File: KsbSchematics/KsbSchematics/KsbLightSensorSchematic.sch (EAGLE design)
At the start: 32 parts, among them IC1 7805L, IC2 LM311N, U1 ATTINY84

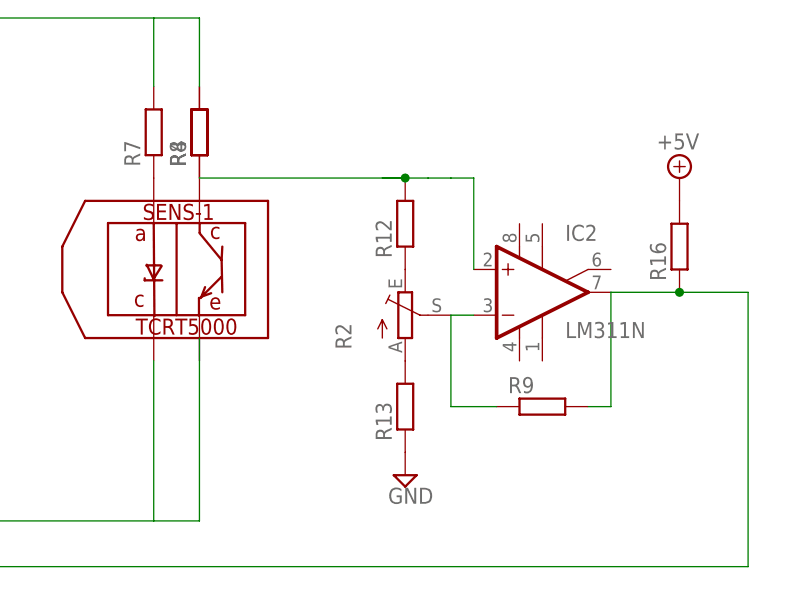
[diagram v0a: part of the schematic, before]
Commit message: minor changes
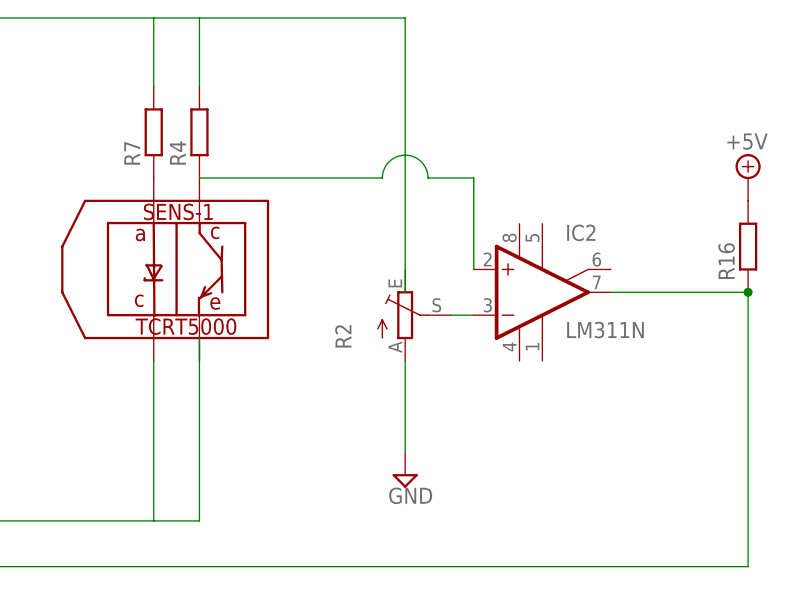
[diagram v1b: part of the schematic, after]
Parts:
- removed R12, R13, R8, R9: (no value), resistor:R-EU_0613/5V
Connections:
- removed net N$14: R4.1, R8.1
- removed net N$17: R12.1, R2.E
- removed net N$18: R13.2, R2.A
- removed net N$7: IC2.-IN, R2.S, R9.1
- new net N$21: IC2.+IN, SENS-1.P$1
- net +12V: no longer R8.2
- net GND: now also R2.A; no longer R13.1
- net N$13: now also IC2.-IN, R2.S; no longer IC2.+IN, R12.2, R8.1, SENS-1.P$1
- net N$4: no longer R9.2
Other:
- moved on the sheet: R16
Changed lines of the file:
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@@
 <part name="R4" library="resistor" deviceset="R-EU_" device="0613/5V"/>
 <part name="R7" library="resistor" deviceset="R-EU_" device="0613/5V"/>
-<part name="R8" library="resistor" deviceset="R-EU_" device="0613/5V"/>
-<part name="R9" library="resistor" deviceset="R-EU_" device="0613/5V"/>
 <part name="R10" library="resistor" deviceset="R-EU_" device="0613/5V" value="2k"/>
 <part name="R11" library="resistor" deviceset="R-EU_" device="0613/5V" value="2k"/>
@@
 <part name="SUPPLY8" library="supply2" deviceset="GND" device=""/>
 <part name="SUPPLY11" library="supply2" deviceset="GND" device=""/>
-<part name="R12" library="resistor" deviceset="R-EU_" device="0613/5V"/>
-<part name="R13" library="resistor" deviceset="R-EU_" device="0613/5V"/>
 <part name="SUPPLY6" library="supply2" deviceset="GND" device=""/>
 <part name="SG1" library="buzzer" deviceset="EFB?" device="AA40D101"/>
@@
 <instance part="R4" gate="G$1" x="93.98" y="152.4" rot="R90"/>
 <instance part="R7" gate="G$1" x="88.9" y="152.4" rot="R90"/>
-<instance part="R8" gate="G$1" x="93.98" y="152.4" rot="R90"/>
-<instance part="R9" gate="G$1" x="132.08" y="121.92"/>
 <instance part="R10" gate="G$1" x="-15.24" y="86.36"/>
 <instance part="R11" gate="G$1" x="-15.24" y="48.26"/>
@@
 <instance part="SUPPLY8" gate="GND" x="-63.5" y="81.28"/>
 <instance part="SUPPLY11" gate="GND" x="-66.04" y="43.18"/>
-<instance part="R12" gate="G$1" x="116.84" y="142.24" rot="R90"/>
-<instance part="R13" gate="G$1" x="116.84" y="121.92" rot="R90"/>
 <instance part="SUPPLY6" gate="GND" x="116.84" y="114.3"/>
 <instance part="SG1" gate="G$1" x="106.68" y="86.36"/>
@@
 <instance part="SUPPLY21" gate="GND" x="10.16" y="0"/>
 <instance part="R15" gate="G$1" x="-12.7" y="7.62"/>
-<instance part="R16" gate="G$1" x="147.32" y="139.7" rot="R90"/>
-<instance part="SUPPLY22" gate="+12V" x="147.32" y="147.32"/>
+<instance part="R16" gate="G$1" x="154.94" y="139.7" rot="R90"/>
+<instance part="SUPPLY22" gate="+12V" x="154.94" y="147.32"/>
 </instances>
 <busses>
@@
 <wire x1="35.56" y1="124.46" x2="35.56" y2="165.1" width="0.1524" layer="91"/>
 <pinref part="R4" gate="G$1" pin="2"/>
-<pinref part="R8" gate="G$1" pin="2"/>
 <wire x1="93.98" y1="165.1" x2="93.98" y2="157.48" width="0.1524" layer="91"/>
 <wire x1="35.56" y1="165.1" x2="88.9" y2="165.1" width="0.1524" layer="91"/>
@@
 <pinref part="R7" gate="G$1" pin="2"/>
 <wire x1="88.9" y1="165.1" x2="88.9" y2="157.48" width="0.1524" layer="91"/>
+<wire x1="93.98" y1="165.1" x2="116.84" y2="165.1" width="0.1524" layer="91"/>
+<wire x1="116.84" y1="165.1" x2="116.84" y2="134.62" width="0.1524" layer="91"/>
 </segment>
 <segment>
@@
 </segment>
 <segment>
-<pinref part="R13" gate="G$1" pin="1"/>
-<pinref part="SUPPLY6" gate="GND" pin="GND"/>
-</segment>
-<segment>
 <pinref part="S3" gate="1" pin="S"/>
 <pinref part="SUPPLY18" gate="GND" pin="GND"/>
@@
 <pinref part="OK1" gate="A" pin="EMIT"/>
 <pinref part="SUPPLY21" gate="GND" pin="GND"/>
+</segment>
+<segment>
+<pinref part="R2" gate="1" pin="A"/>
+<pinref part="SUPPLY6" gate="GND" pin="GND"/>
+<wire x1="116.84" y1="127" x2="116.84" y2="116.84" width="0.1524" layer="91"/>
 </segment>
 </net>
@@
 </segment>
 </net>
-<net name="N$13" class="0">
-<segment>
-<wire x1="93.98" y1="147.32" x2="116.84" y2="147.32" width="0.1524" layer="91"/>
-<wire x1="116.84" y1="147.32" x2="114.3" y2="147.32" width="0.1524" layer="91"/>
-<wire x1="121.92" y1="147.32" x2="124.46" y2="147.32" width="0.1524" layer="91"/>
-<wire x1="124.46" y1="147.32" x2="124.46" y2="137.16" width="0.1524" layer="91"/>
-<wire x1="116.84" y1="147.32" x2="119.38" y2="147.32" width="0.1524" layer="91"/>
-<wire x1="121.92" y1="147.32" x2="119.38" y2="147.32" width="0.1524" layer="91"/>
-<junction x="116.84" y="147.32"/>
-<pinref part="SENS-1" gate="G$1" pin="P$1"/>
-<pinref part="R8" gate="G$1" pin="1"/>
-<pinref part="R12" gate="G$1" pin="2"/>
-<pinref part="IC2" gate="A" pin="+IN"/>
-</segment>
-</net>
-<net name="N$14" class="0">
-<segment>
-<pinref part="R4" gate="G$1" pin="1"/>
-<pinref part="R8" gate="G$1" pin="1"/>
-</segment>
-</net>
 <net name="N$4" class="0">
 <segment>
@@
 <wire x1="154.94" y1="104.14" x2="30.48" y2="104.14" width="0.1524" layer="91"/>
 <wire x1="154.94" y1="134.62" x2="154.94" y2="104.14" width="0.1524" layer="91"/>
-<wire x1="139.7" y1="134.62" x2="147.32" y2="134.62" width="0.1524" layer="91"/>
-<wire x1="147.32" y1="134.62" x2="154.94" y2="134.62" width="0.1524" layer="91"/>
-<wire x1="139.7" y1="134.62" x2="139.7" y2="121.92" width="0.1524" layer="91"/>
-<wire x1="139.7" y1="121.92" x2="137.16" y2="121.92" width="0.1524" layer="91"/>
+<wire x1="139.7" y1="134.62" x2="154.94" y2="134.62" width="0.1524" layer="91"/>
 <wire x1="30.48" y1="73.66" x2="35.56" y2="73.66" width="0.1524" layer="91"/>
 <wire x1="30.48" y1="81.28" x2="30.48" y2="73.66" width="0.1524" layer="91" curve="180"/>
 <pinref part="IC2" gate="A" pin="OUT"/>
-<pinref part="R9" gate="G$1" pin="2"/>
 <pinref part="R16" gate="G$1" pin="1"/>
-<junction x="147.32" y="134.62"/>
-</segment>
-</net>
-<net name="N$7" class="0">
-<segment>
-<wire x1="121.92" y1="132.08" x2="124.46" y2="132.08" width="0.1524" layer="91"/>
-<wire x1="127" y1="121.92" x2="121.92" y2="121.92" width="0.1524" layer="91"/>
-<wire x1="121.92" y1="121.92" x2="121.92" y2="132.08" width="0.1524" layer="91"/>
-<pinref part="R9" gate="G$1" pin="1"/>
-<pinref part="IC2" gate="A" pin="-IN"/>
-<pinref part="R2" gate="1" pin="S"/>
+<junction x="154.94" y="134.62"/>
 </segment>
 </net>
@@
 </segment>
 </net>
-<net name="N$17" class="0">
-<segment>
-<pinref part="R2" gate="1" pin="E"/>
-<pinref part="R12" gate="G$1" pin="1"/>
-</segment>
-</net>
-<net name="N$18" class="0">
-<segment>
-<pinref part="R2" gate="1" pin="A"/>
-<pinref part="R13" gate="G$1" pin="2"/>
-</segment>
-</net>
 <net name="N$5" class="0">
 <segment>
@@
 </segment>
 </net>
+<net name="N$21" class="0">
+<segment>
+<wire x1="114.3" y1="147.32" x2="119.38" y2="147.32" width="0.1524" layer="91" curve="-180"/>
+<wire x1="124.46" y1="147.32" x2="124.46" y2="137.16" width="0.1524" layer="91"/>
+<pinref part="IC2" gate="A" pin="+IN"/>
+<wire x1="119.38" y1="147.32" x2="124.46" y2="147.32" width="0.1524" layer="91"/>
+<pinref part="SENS-1" gate="G$1" pin="P$1"/>
+<wire x1="114.3" y1="147.32" x2="93.98" y2="147.32" width="0.1524" layer="91"/>
+</segment>
+</net>
+<net name="N$13" class="0">
+<segment>
+<pinref part="IC2" gate="A" pin="-IN"/>
+<wire x1="121.92" y1="132.08" x2="124.46" y2="132.08" width="0.1524" layer="91"/>
+<pinref part="R2" gate="1" pin="S"/>
+</segment>
+</net>
